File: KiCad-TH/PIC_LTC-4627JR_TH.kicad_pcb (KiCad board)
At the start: 2 copper layers, 0 parts

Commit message: PCB Routing Round 5 Begins
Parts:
- added J1: Conn_01x05_Male, Pin_Headers:Pin_Header_Straight_1x05_Pitch2.54mm, F.Cu at (95.9, 113.7)
- added J2: Conn_01x04, Connectors_JST:JST_PH_B4B-PH-K_04x2.00mm_Straight, F.Cu at (104.1, 119.4)
- added L1: LTC-4627JR, LTC-4627JR:LTC-4627JR, F.Cu at (114.5, 83.8)
- added Q1: Q_NPN_EBC, TO_SOT_Packages_THT:TO-92_Inline_Narrow_Oval, F.Cu at (119.4, 95.2)
- added Q2: Q_NPN_EBC, TO_SOT_Packages_THT:TO-92_Inline_Narrow_Oval, F.Cu at (100.3, 95.2)
- added Q3: Q_NPN_EBC, TO_SOT_Packages_THT:TO-92_Inline_Narrow_Oval, F.Cu at (125.7, 95.2)
- added Q4: Q_NPN_EBC, TO_SOT_Packages_THT:TO-92_Inline_Narrow_Oval, F.Cu at (113.0, 95.2)
- added Q5: Q_NPN_EBC, TO_SOT_Packages_THT:TO-92_Inline_Narrow_Oval, F.Cu at (106.7, 95.2)
- added R1: 120, Resistors_THT:R_Axial_DIN0207_L6.3mm_D2.5mm_P10.16mm_Horizontal, F.Cu at (98.4, 99.1)
- added R10: 1k, Resistors_THT:R_Axial_DIN0207_L6.3mm_D2.5mm_P10.16mm_Horizontal, F.Cu at (114.3, 99.1)
- added R11: 1k, Resistors_THT:R_Axial_DIN0207_L6.3mm_D2.5mm_P10.16mm_Horizontal, F.Cu at (130.2, 99.1)
- added R12: 1k, Resistors_THT:R_Axial_DIN0207_L6.3mm_D2.5mm_P10.16mm_Horizontal, F.Cu at (104.8, 99.1)
- added R13: 1k, Resistors_THT:R_Axial_DIN0207_L6.3mm_D2.5mm_P10.16mm_Horizontal, F.Cu at (123.8, 99.1)
- added R2: 120, Resistors_THT:R_Axial_DIN0207_L6.3mm_D2.5mm_P10.16mm_Horizontal, F.Cu at (133.3, 99.1)
- added R3: 120, Resistors_THT:R_Axial_DIN0207_L6.3mm_D2.5mm_P10.16mm_Horizontal, F.Cu at (120.7, 99.1)
- added R4: 120, Resistors_THT:R_Axial_DIN0207_L6.3mm_D2.5mm_P10.16mm_Horizontal, F.Cu at (111.1, 99.1)
- added R5: 120, Resistors_THT:R_Axial_DIN0207_L6.3mm_D2.5mm_P10.16mm_Horizontal, F.Cu at (117.5, 99.1)
- added R6: 120, Resistors_THT:R_Axial_DIN0207_L6.3mm_D2.5mm_P10.16mm_Horizontal, F.Cu at (95.2, 99.1)
- added R7: 120, Resistors_THT:R_Axial_DIN0207_L6.3mm_D2.5mm_P10.16mm_Horizontal, F.Cu at (101.6, 99.1)
- added R8: 120, Resistors_THT:R_Axial_DIN0207_L6.3mm_D2.5mm_P10.16mm_Horizontal, F.Cu at (127.0, 99.1)
- added R9: 1k, Resistors_THT:R_Axial_DIN0207_L6.3mm_D2.5mm_P10.16mm_Horizontal, F.Cu at (108.0, 99.1)
- added U1: PIC16F18344-P, Housings_DIP:DIP-20_W7.62mm, F.Cu at (109.9, 121.3)

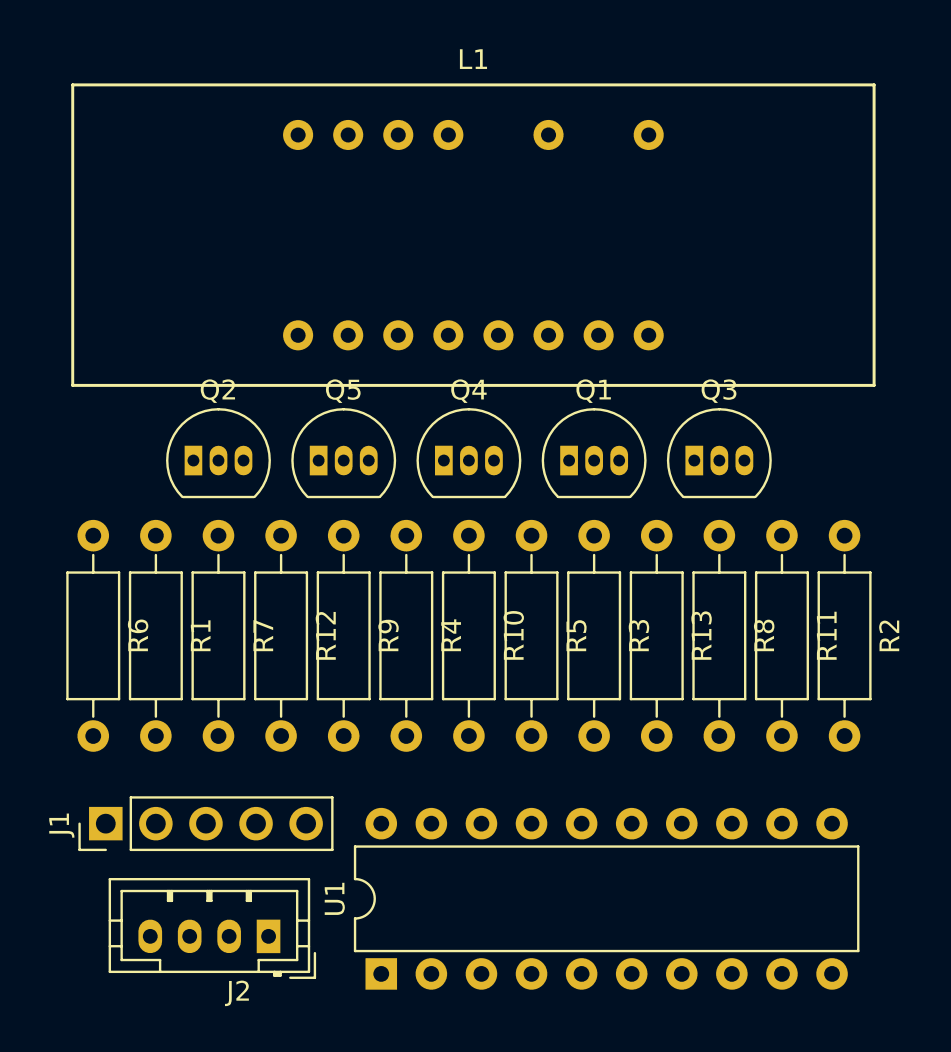
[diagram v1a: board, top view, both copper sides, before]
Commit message: PCB #5 Looking Good Still Needs Polish
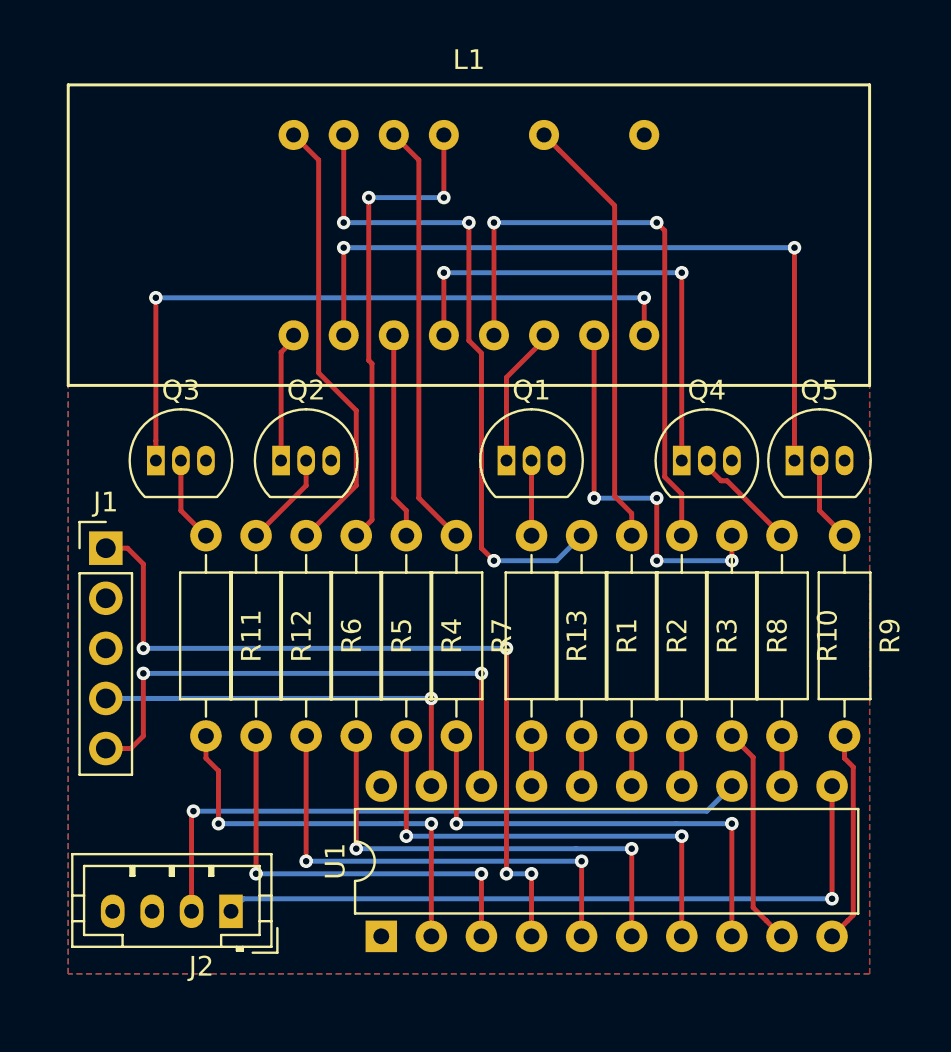
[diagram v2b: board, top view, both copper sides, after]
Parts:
- moved R11 29.2 mm to (101.0, 99.1)
- moved Q3 27.3 mm to (98.4, 95.2)
- moved R9 25.4 mm to (133.3, 99.1)
- moved Q5 24.1 mm to (130.8, 95.2)
- moved R1 21.6 mm to (120.0, 99.1)
- moved R10 15.9 mm to (130.2, 99.1)
- moved J1 14.0 mm to (95.9, 99.7), turned to 0 degrees
- moved R7 12.1 mm to (113.7, 99.1)
- moved Q4 12.1 mm to (125.1, 95.2)
- moved R6 10.8 mm to (106.0, 99.1)
- moved R2 10.8 mm to (122.6, 99.1)
- moved R5 8.89 mm to (108.6, 99.1)
- moved R13 6.35 mm to (117.5, 99.1)
- moved Q2 4.45 mm to (104.8, 95.2)
- moved R3 4.44 mm to (125.1, 99.1)
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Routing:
- net /VPP: track 0.00 -> 40.8 mm, vias 0 -> 4
- net /DIG_2: track 0.00 -> 38.1 mm, vias 0 -> 2
- net /I2CCL: track 0.00 -> 36.5 mm, vias 0 -> 1
- net /DIG_4: track 0.00 -> 34.9 mm, vias 0 -> 2
- net Net-(L1-Pad15): track 0.00 -> 33.4 mm, vias 0 -> 3
- net /I2CDA: track 0.00 -> 32.2 mm, vias 0 -> 1
- net Net-(L1-Pad5): track 0.00 -> 30.4 mm, vias 0 -> 2
- net /ICSPCLK: track 0.00 -> 28.2 mm, vias 0 -> 2
- net /DIG_L: track 0.00 -> 24.8 mm, vias 0 -> 2
- net Net-(L1-Pad13): track 0.00 -> 24.5 mm, vias 0 -> 2
- net Net-(R5-Pad2): track 0.00 -> 24.1 mm, vias 0 -> 2
- net Net-(R7-Pad2): track 0.00 -> 24.1 mm, vias 0 -> 2
- net Net-(R6-Pad2): track 0.00 -> 24.1 mm, vias 0 -> 2
- net Net-(R4-Pad2): track 0.00 -> 24.1 mm, vias 0 -> 2
- net Net-(L1-Pad16): track 0.00 -> 22.7 mm
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- added copper zone on F.Cu, net GND
- added copper zone on B.Cu, net VCC
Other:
- net class Default: trace_width 0.1524 -> 0.25
